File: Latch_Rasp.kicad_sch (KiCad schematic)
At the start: 18 parts, among them J2 Conn_02x03_Counter_Clockwise, J5 USB_C_Receptacle_PowerOnly_6P, Q1 NDT456P, Q2 AO3414, SW1 SW_Push

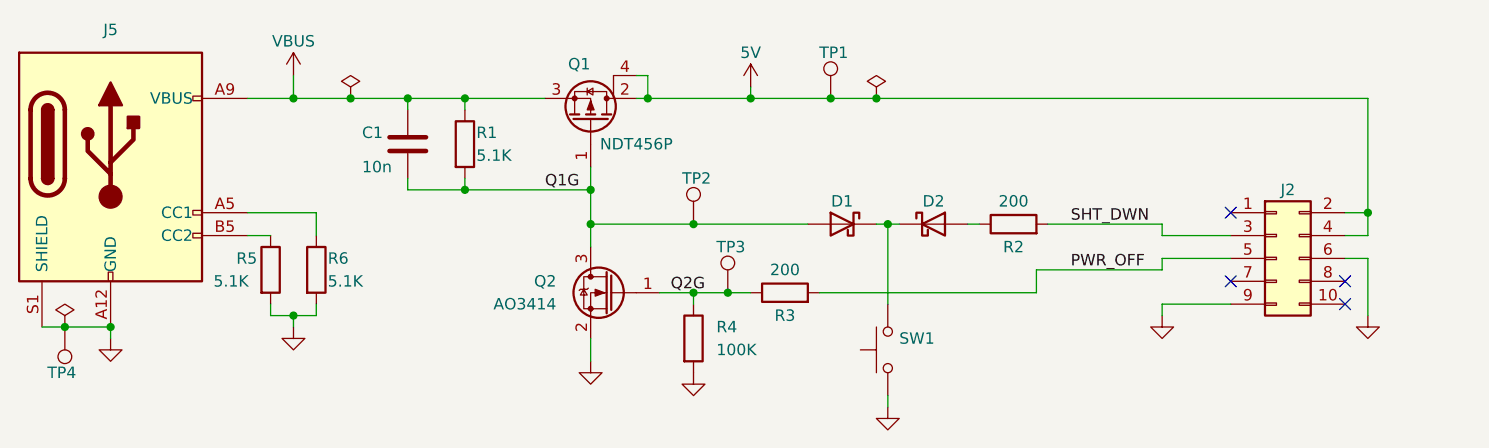
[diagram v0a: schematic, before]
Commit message: wip
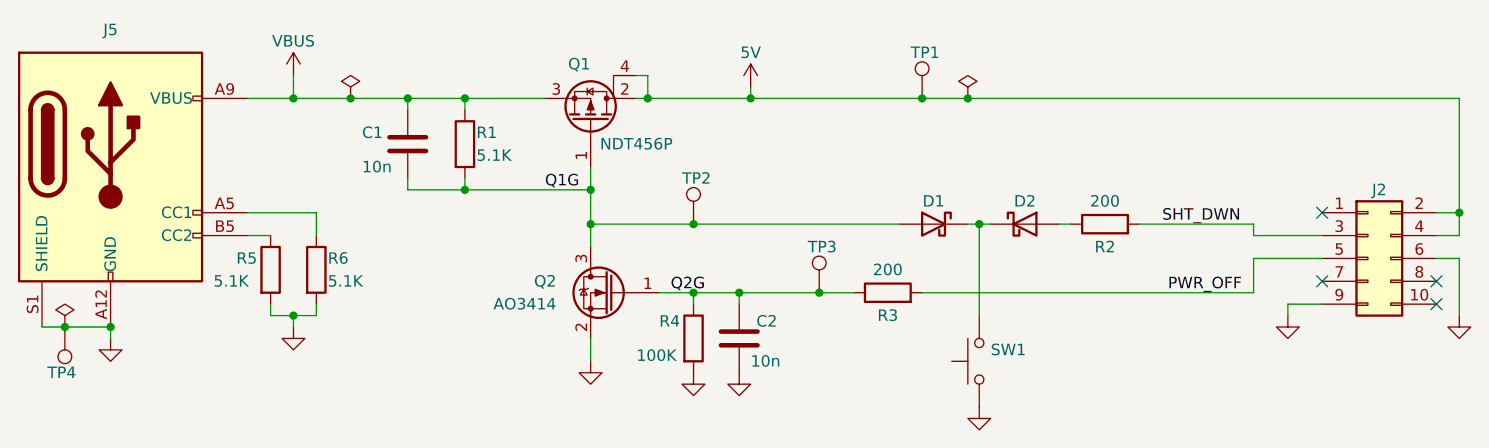
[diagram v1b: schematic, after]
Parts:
- added C2: 10n, Capacitor_SMD:C_0805_2012Metric, symbol Device:C
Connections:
- net GND: now also C2.2
- net Q2G: now also C2.1
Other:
- moved on the sheet: D1, D2, J2, R2, R3, SW1, TP1, TP3
